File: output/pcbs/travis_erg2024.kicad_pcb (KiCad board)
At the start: 2 copper layers, 406.4 x 146.4 mm, 197 parts

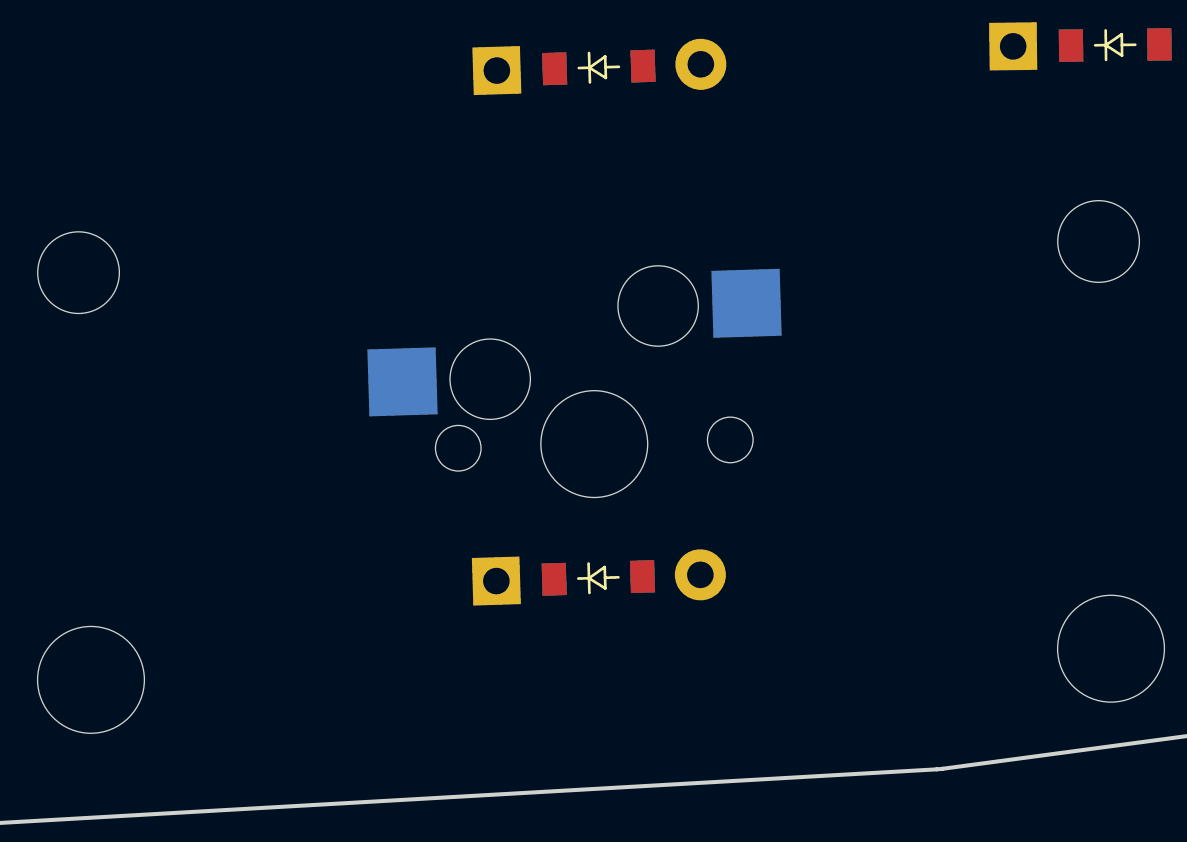
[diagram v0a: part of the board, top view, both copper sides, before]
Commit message: 3d adjustments
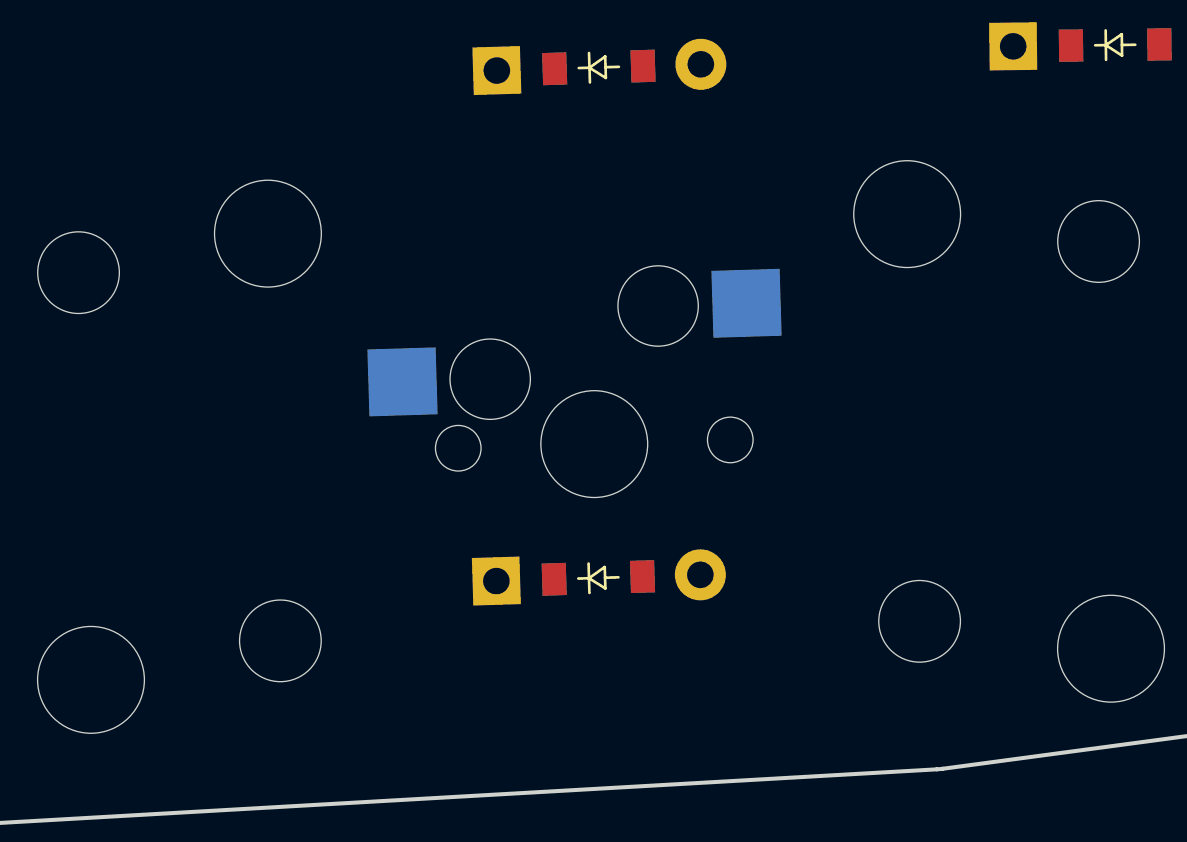
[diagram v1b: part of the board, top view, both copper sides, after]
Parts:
- STAB2u2: value MX_Stabilizer_Cutout-2u -> Stabilizer_MX_2.00u; footprint MX_Stabilizer_Cutout-2u -> Stabilizer_MX_2.00u
- turned STAB2u2 to 181.75 degrees
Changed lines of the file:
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@@
     )
   )
-    (module MX_Stabilizer_Cutout-2u (layer F.Cu)
-    (at 192.703245 170.1296884 1.75)
-    (fp_text reference "STAB2u2" (at 0.25 10.05) (layer Eco2.User) hide hide
+    (module Stabilizer_MX_2.00u (layer F.Cu)
+    (descr "MX PCB Stabilizer 2.00u 2.25u 2.50u 2.75u")
+    (tags "MX Keyboard Stabilizer 2.00u 2.25u 2.50u 2.75u Cutout")
+    (at 192.703245 170.1296884 181.75)
+    (attr virtual)
+    (fp_text reference "STAB2u2" (at 0 -2) (layer F.SilkS) hide
       (effects (font (size 1 1) (thickness 0.15)))
     )
-    (fp_text value MX_Stabilizer_Cutout-2u (at 0 -15.24) (layer F.Fab) hide
+    (fp_text value Stabilizer_MX_2.00u (at 0 2) (layer F.Fab)
       (effects (font (size 1 1) (thickness 0.15)))
     )
-    (fp_line (start -19 -9.5) (end 19 -9.5) (layer Dwgs.User) (width 0.15))
-    (fp_line (start -19 9.5) (end -19 -9.5) (layer Dwgs.User) (width 0.15))
-    (fp_line (start 19 9.5) (end -19 9.5) (layer Dwgs.User) (width 0.15))
-    (fp_line (start 19 -9.5) (end 19 9.5) (layer Dwgs.User) (width 0.15))
-    (pad "" np_thru_hole oval (at 11.938 7.7724) (size 3.048 0.3048) (drill oval 3.048 0.3048) (layers *.Cu *.Mask))
-    (pad "" np_thru_hole oval (at 11.938 -5.5372) (size 6.6548 0.3048) (drill oval 6.6548 0.3048) (layers *.Cu *.Mask))
-    (pad "" np_thru_hole oval (at 8.763 0.4572) (size 0.3048 12.2936) (drill oval 0.3048 12.2936) (layers *.Cu *.Mask))
-    (pad "" np_thru_hole oval (at 11.938 6.4516) (size 6.6548 0.3048) (drill oval 6.6548 0.3048) (layers *.Cu *.Mask))
-    (pad "" np_thru_hole oval (at 15.113 0.4572) (size 0.3048 12.2936) (drill oval 0.3048 12.2936) (layers *.Cu *.Mask))
-    (pad "" np_thru_hole oval (at 15.9766 -0.889) (size 0.3048 2.794) (drill oval 0.3048 2.794) (layers *.Cu *.Mask))
-    (pad "" np_thru_hole oval (at 10.5664 7.112) (size 0.3048 1.4732) (drill oval 0.3048 1.4732) (layers *.Cu *.Mask))
-    (pad "" np_thru_hole oval (at 15.5448 -2.1336) (size 1.1684 0.3048) (drill oval 1.1684 0.3048) (layers *.Cu *.Mask))
-    (pad "" np_thru_hole oval (at 13.3096 7.112) (size 0.3048 1.4732) (drill oval 0.3048 1.4732) (layers *.Cu *.Mask))
-    (pad "" np_thru_hole oval (at 15.5448 0.3556) (size 1.1684 0.3048) (drill oval 1.1684 0.3048) (layers *.Cu *.Mask))
-    (pad "" np_thru_hole oval (at -11.938 -5.5372) (size 6.6548 0.3048) (drill oval 6.6548 0.3048) (layers *.Cu *.Mask))
-    (pad "" np_thru_hole oval (at -15.5448 -2.1336) (size 1.1684 0.3048) (drill oval 1.1684 0.3048) (layers *.Cu *.Mask))
-    (pad "" np_thru_hole oval (at -15.9766 -0.889) (size 0.3048 2.794) (drill oval 0.3048 2.794) (layers *.Cu *.Mask))
-    (pad "" np_thru_hole oval (at -15.113 0.4572) (size 0.3048 12.2936) (drill oval 0.3048 12.2936) (layers *.Cu *.Mask))
-    (pad "" np_thru_hole oval (at -8.763 0.4572) (size 0.3048 12.2936) (drill oval 0.3048 12.2936) (layers *.Cu *.Mask))
-    (pad "" np_thru_hole oval (at -11.938 6.4516) (size 6.6548 0.3048) (drill oval 6.6548 0.3048) (layers *.Cu *.Mask))
-    (pad "" np_thru_hole oval (at -15.5448 0.3556) (size 1.1684 0.3048) (drill oval 1.1684 0.3048) (layers *.Cu *.Mask))
-    (pad "" np_thru_hole oval (at -13.3096 7.112) (size 0.3048 1.4732) (drill oval 0.3048 1.4732) (layers *.Cu *.Mask))
-    (pad "" np_thru_hole oval (at -10.5664 7.112) (size 0.3048 1.4732) (drill oval 0.3048 1.4732) (layers *.Cu *.Mask))
-    (pad "" np_thru_hole oval (at -11.938 7.7724) (size 3.048 0.3048) (drill oval 3.048 0.3048) (layers *.Cu *.Mask))
+    (fp_line (start 0 2) (end 0 -2) (layer Dwgs.User) (width 0.1))
+    (fp_line (start -2 0) (end 2 0) (layer Dwgs.User) (width 0.1))
+    (fp_line (start 8.563 -5.53) (end 8.563 6.77) (layer Eco1.User) (width 0.1))
+    (fp_line (start 8.563 6.77) (end 15.313 6.77) (layer Eco1.User) (width 0.1))
+    (fp_line (start 15.313 6.77) (end 15.313 -5.53) (layer Eco1.User) (width 0.1))
+    (fp_line (start 15.313 -5.53) (end 8.563 -5.53) (layer Eco1.User) (width 0.1))
+    (fp_line (start -15.313 -5.53) (end -15.313 6.77) (layer Eco1.User) (width 0.1))
+    (fp_line (start -15.313 6.77) (end -8.563 6.77) (layer Eco1.User) (width 0.1))
+    (fp_line (start -8.563 6.77) (end -8.563 -5.53) (layer Eco1.User) (width 0.1))
+    (fp_line (start -8.563 -5.53) (end -15.313 -5.53) (layer Eco1.User) (width 0.1))
+    (pad "" np_thru_hole circle (at -11.938 -6.985) (size 3.048 3.048) (drill 3.048) (layers *.Cu *.Mask))
+    (pad "" np_thru_hole circle (at 11.938 -6.985) (size 3.048 3.048) (drill 3.048) (layers *.Cu *.Mask))
+    (pad "" np_thru_hole circle (at -11.938 8.225) (size 3.9878 3.9878) (drill 3.9878) (layers *.Cu *.Mask))
+    (pad "" np_thru_hole circle (at 11.938 8.225) (size 3.9878 3.9878) (drill 3.9878) (layers *.Cu *.Mask))
+    (fp_text user %R (at 0 0) (layer F.Fab)
+      (effects (font (size 1 1) (thickness 0.15)))
+    )
+    (model ${SCOTTOKEEBS_KICAD}/3dmodels/ScottoKeebs_Stabilizer.3dshapes/Stabilizer_MX_2.00u.step
+      (at (xyz 0 0 0))
+      (scale (xyz 1 1 1))
+      (rotate (xyz 0 0 0))
+    )
   )
     (module Stabilizer_MX_3.00u (layer F.Cu)
